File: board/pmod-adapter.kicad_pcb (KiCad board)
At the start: 2 copper layers, 20.3 x 86.4 mm, 4 parts

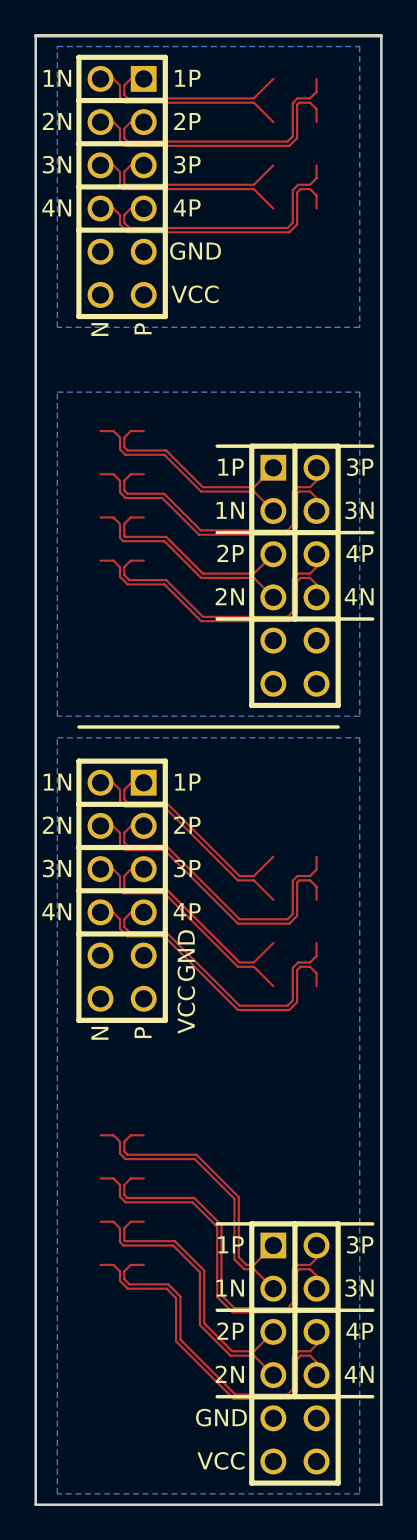
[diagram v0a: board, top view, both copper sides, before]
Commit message: Length matching.
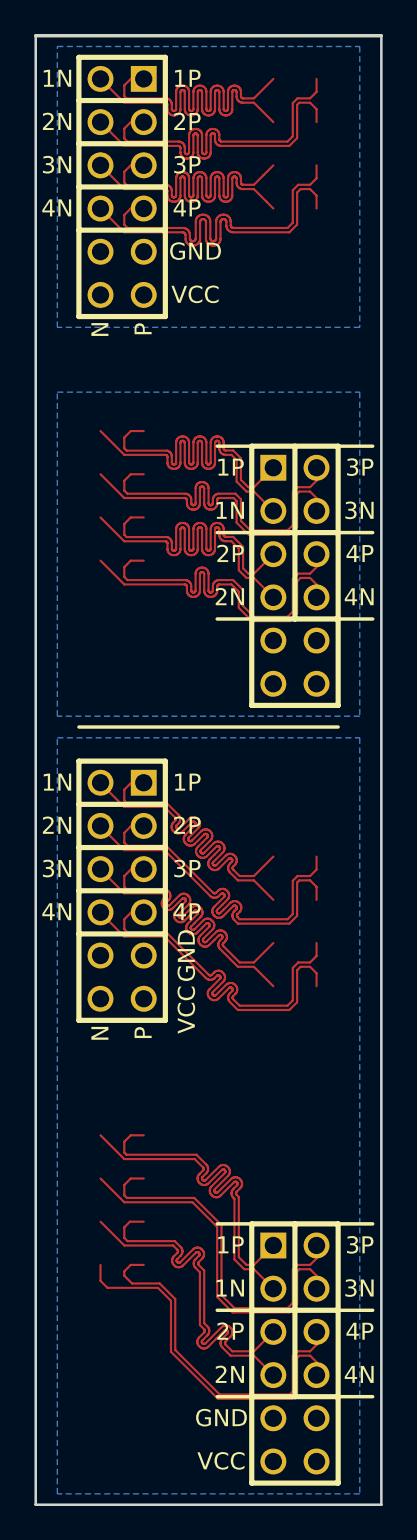
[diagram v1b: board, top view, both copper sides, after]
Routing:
- net /J1A_P: track 11.2 -> 21.3 mm
- net /J1C_P: track 11.3 -> 21.2 mm
- net /J1A_N: track 11.6 -> 21.3 mm
- net /J1C_N: track 11.7 -> 21.2 mm
- net /J2A_P: track 12.1 -> 21.3 mm
- net /J2C_P: track 12.2 -> 21.2 mm
- net /J2A_N: track 12.5 -> 21.3 mm
- net /J2C_N: track 12.6 -> 21.2 mm
- net /J3A_P: track 13.0 -> 21.3 mm
- net /J3C_P: track 13.1 -> 21.2 mm
- net /J3A_N: track 13.4 -> 21.3 mm
- net /J3C_N: track 13.5 -> 21.2 mm
- net /J4C_P: track 15.8 -> 21.2 mm
- net /J4A_P: track 15.9 -> 21.3 mm
- net /J1D_P: track 16.3 -> 21.3 mm
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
